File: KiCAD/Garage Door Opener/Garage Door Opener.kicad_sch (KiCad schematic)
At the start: 8 parts, among them J1 Screw_Terminal_01x03, J3 Conn_01x02_Pin, K1 JQC-3FF-S-Z, Q1 S8550, SW1 SW_Push_Dual, U1 ESP32-S3-DevKitC

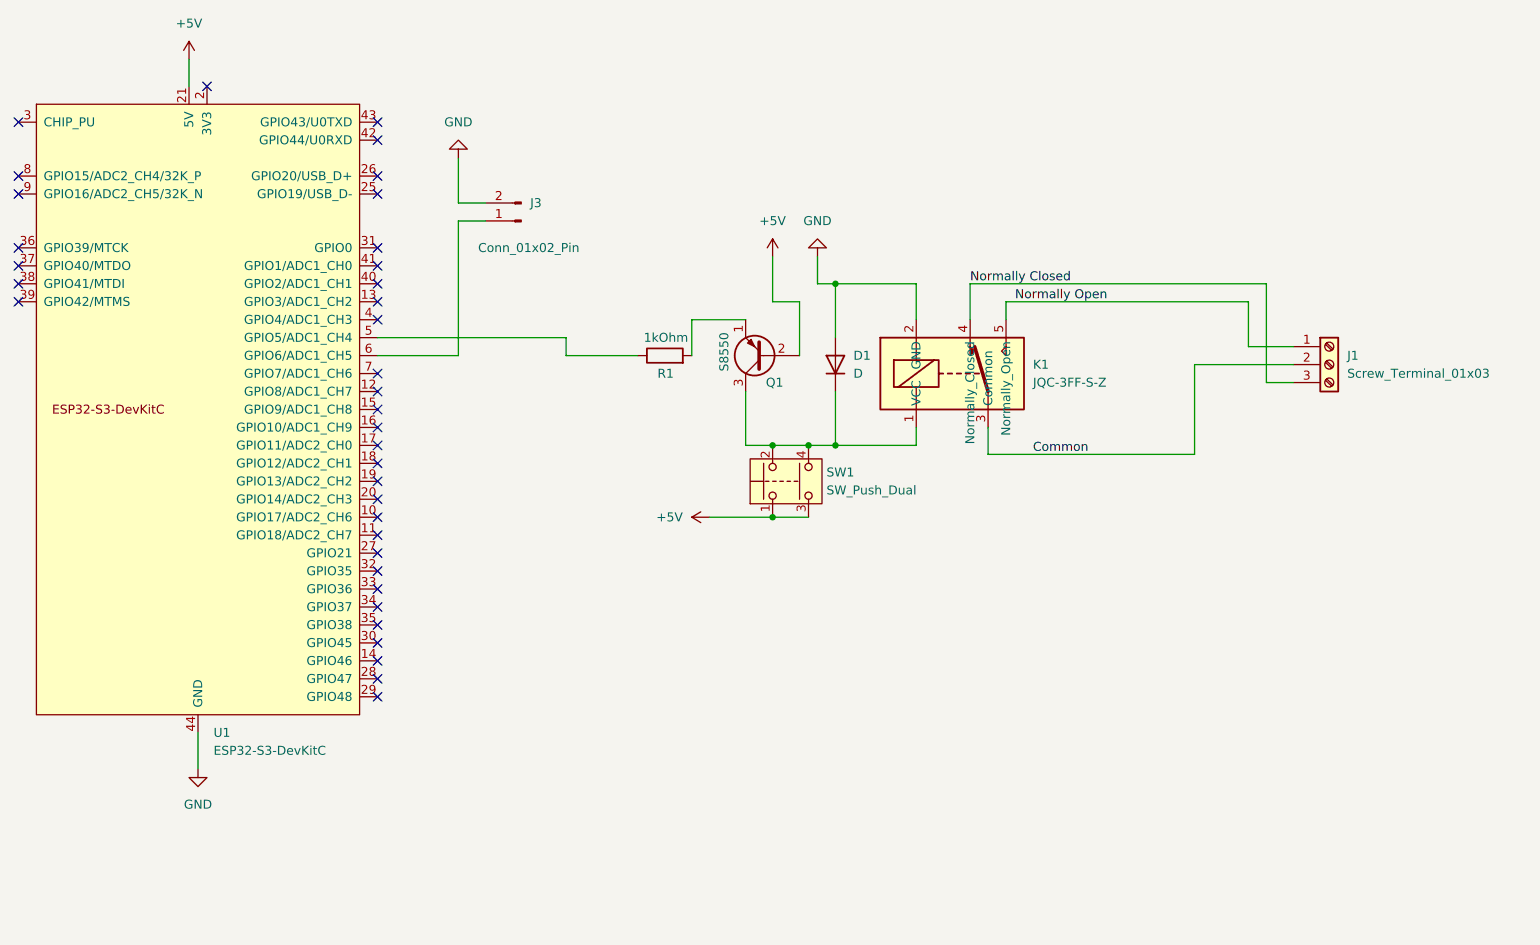
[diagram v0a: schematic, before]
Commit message: Updated board design
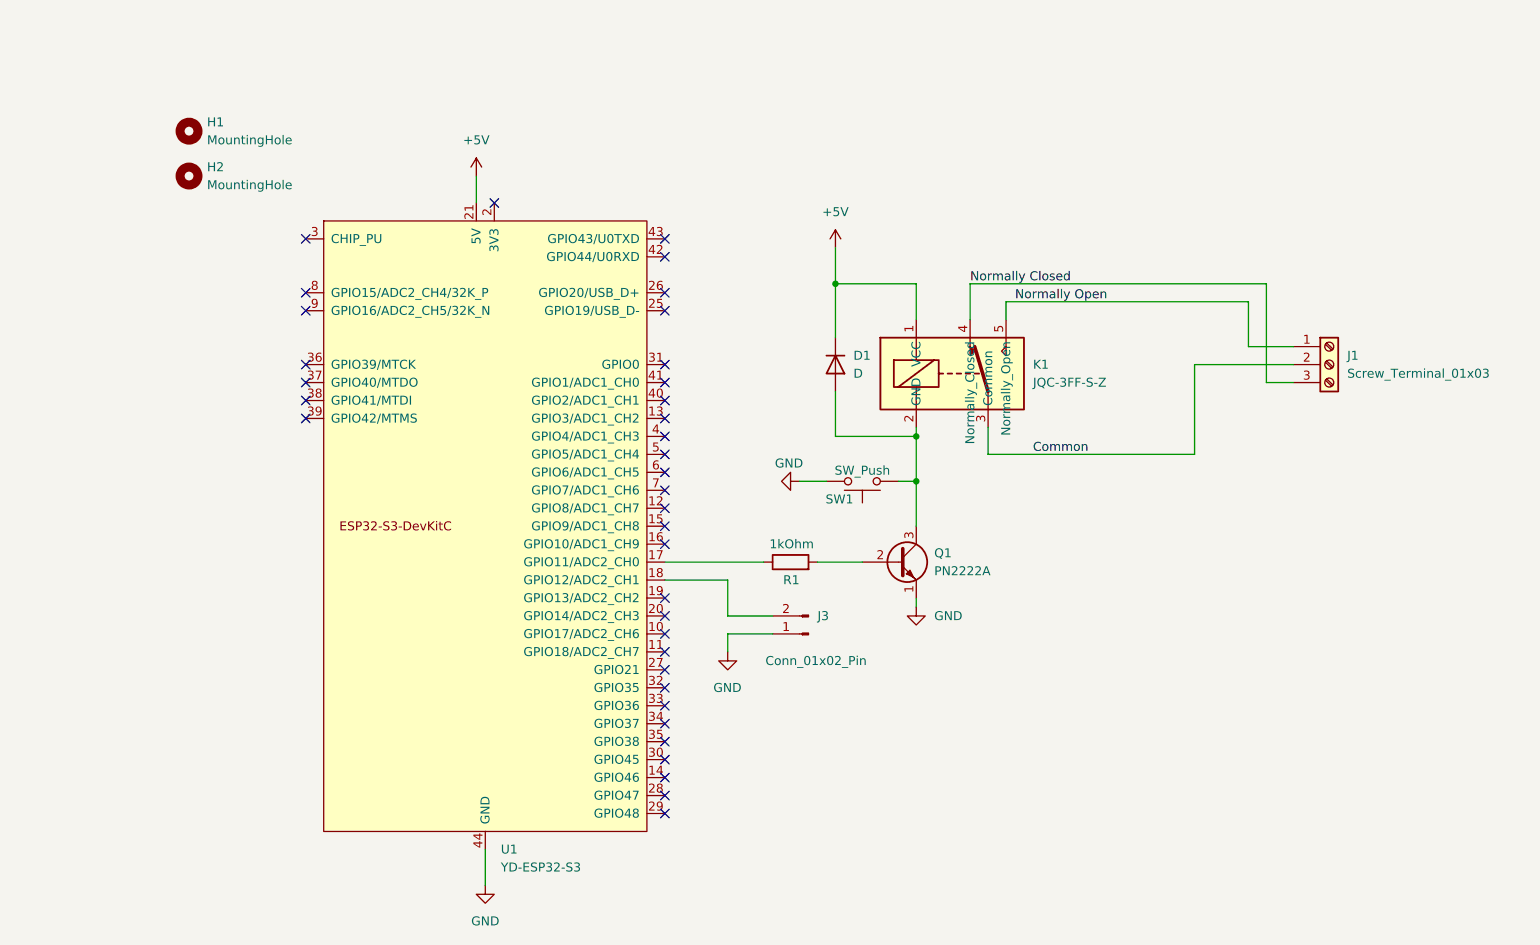
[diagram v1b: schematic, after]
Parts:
- removed Q1: S8550, Package_TO_SOT_SMD:SOT-23, symbol Transistor_BJT:S8550
- added H1, H2: MountingHole, MountingHole:MountingHole_3.5mm, symbol Mechanical:MountingHole
- added Q1: PN2222A, Package_TO_SOT_THT:TO-92_Inline, symbol Transistor_BJT:PN2222A
- SW1: value SW_Push_Dual -> SW_Push; symbol Switch:SW_Push_Dual -> Switch:SW_Push
- U1: value ESP32-S3-DevKitC -> YD-ESP32-S3
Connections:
- net +5V: now also D1.1 (K), K1.1 (VCC); no longer SW1.1, SW1.3
- net GND: now also J3.1 (Pin_1), SW1.2, Q1.1 (E); no longer D1.2 (A), J3.2 (Pin_2), K1.2 (GND)
- net at U1.17 (GPIO11/ADC2_CH0): now also R1.1
- net at U1.18 (GPIO12/ADC2_CH1): now also J3.2 (Pin_2)
- net at U1.5 (GPIO5/ADC1_CH4): no longer R1.1
- net at U1.6 (GPIO6/ADC1_CH5): no longer J3.1 (Pin_1)
- net at R1.2: now also Q1.2 (B)
- new net: D1.2 (A), K1.2 (GND), Q1.3 (C), SW1.1
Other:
- moved on the sheet: D1, J3, R1, U1
